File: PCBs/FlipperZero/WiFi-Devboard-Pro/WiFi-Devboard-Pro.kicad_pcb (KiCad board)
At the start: 2 copper layers, 78.5 x 20.1 mm, 46 parts, among them IC1 ESP32-WROOM-32E-N4, IC2 DMP1045U-7, IC3 AZ1117H-3.3TRE1, IC4 DMP1045U-7, IC5 DMP1045U-7, J1 3220-10-0300-00, J2 X6511WVS-08H-C60D48R2, J3 DZ254S-11-10-48, J4 Conn_01x11, J5 Conn_01x11, J6 503398-1892, U1 MMDT2907A-7-F, U2 MMDT2907A-7-F, U3 MMDT2907A-7-F

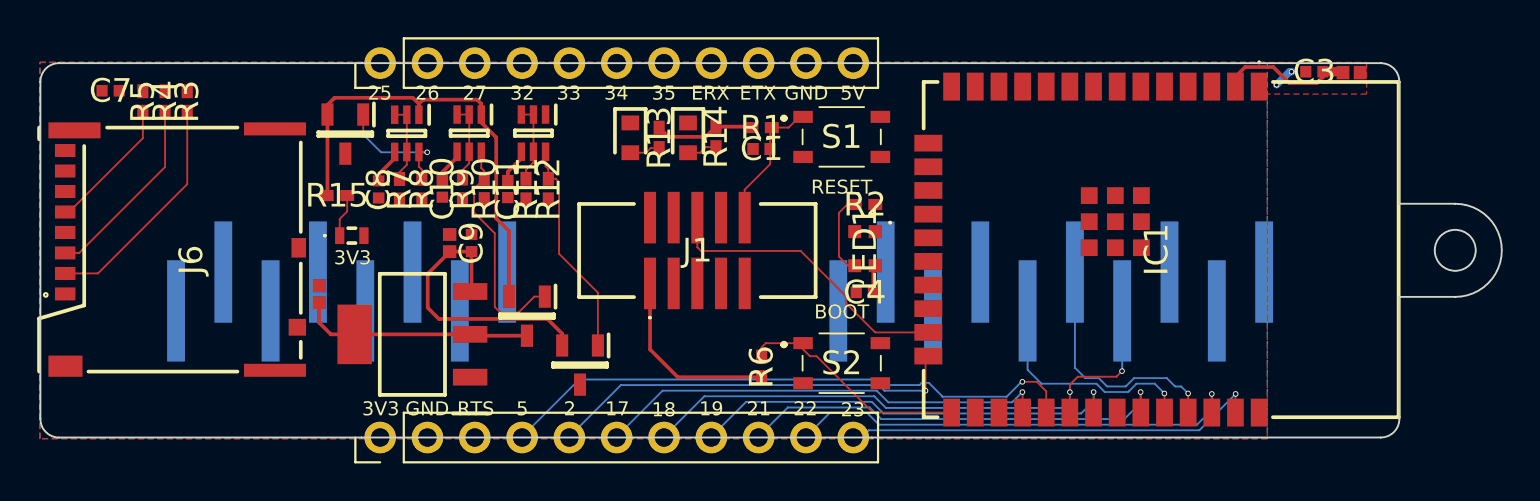
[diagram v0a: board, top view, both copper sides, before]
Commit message: Finish all but one connection
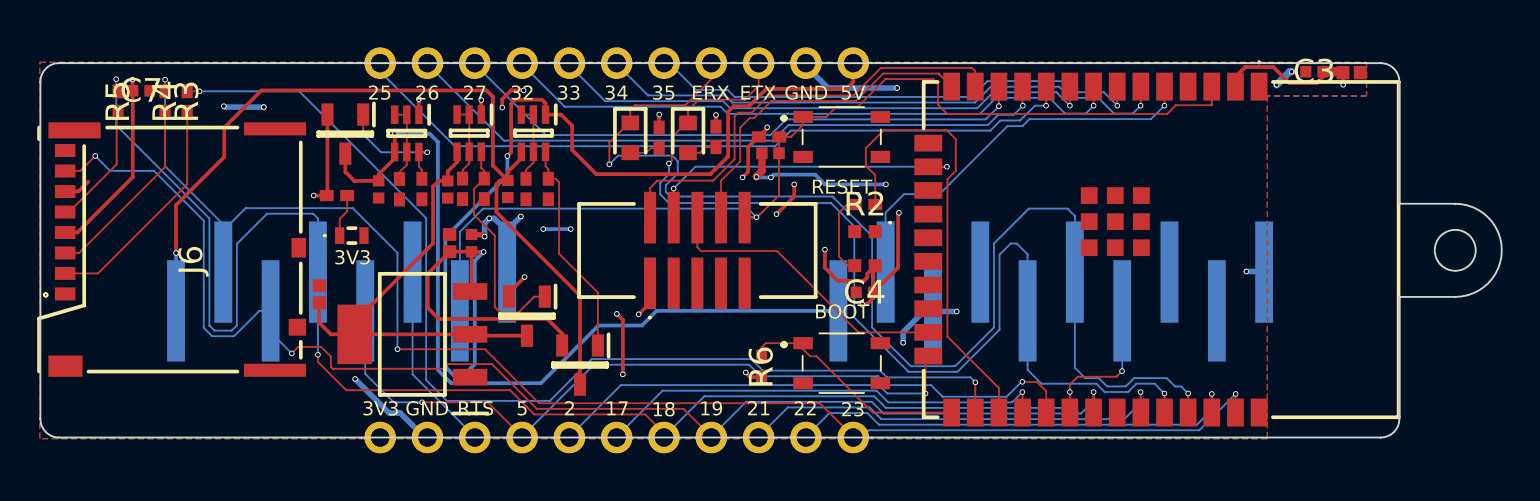
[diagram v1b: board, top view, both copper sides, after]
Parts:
- moved C7 1.65 mm to (116.5, 91.3), turned to 180 degrees
- moved R5 1.33 mm to (115.3, 91.9)
- moved R1 0.64 mm to (150.2, 93.8)
- moved C1 0.53 mm to (150.3, 94.7)
- moved C10 0.29 mm to (133.0, 96.6)
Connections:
- C4 pad 2: +5V -> +3V3
- LED1 pad 4: +5V -> +3V3
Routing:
- net GPIO04: track 0.00 -> 57.4 mm, vias 0 -> 2
- net GPIO23: track 22.5 -> 79.4 mm, vias 1 -> 3
- net GPIO18: track 31.5 -> 86.7 mm, vias 2 -> 4
- net RX: track 13.2 -> 66.4 mm, vias 1 -> 2
- net +5V: track 16.8 -> 65.4 mm, vias 0 -> 2
- net GPIO19: track 23.4 -> 70.7 mm, vias 1 -> 3
- net RESET: track 7.35 -> 54.6 mm, vias 0 -> 1
- net TX: track 12.5 -> 58.2 mm, vias 1 -> 2
- net +ext_5V: track 2.22 -> 46.7 mm, vias 0 -> 1
- net +ext_3V3: track 1.91 -> 44.0 mm, vias 0 -> 1
- net GPIO25: track 0.00 -> 39.7 mm, vias 0 -> 1
- net GND: track 1.09 -> 38.8 mm, vias 2 -> 17
- net GPIO26: track 0.00 -> 35.5 mm, vias 0 -> 1
- net GPIO32: track 0.00 -> 33.7 mm, vias 0 -> 1
- net GPIO27: track 0.00 -> 31.4 mm, vias 0 -> 1
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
